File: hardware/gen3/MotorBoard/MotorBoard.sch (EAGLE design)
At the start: 245 parts, among them M10O1 TEST_PT, M1O2 TEST_PT, M1O3 TEST_PT, M2O1 TEST_PT, M2O2 TEST_PT, M2O3 TEST_PT, M3O1 TEST_PT, M3O2 TEST_PT, M3O3 TEST_PT, M4O1 TEST_PT, M4O2 TEST_PT, M4O3 TEST_PT, U2 ATMEGA165PV-8AU

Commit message: fixed weird package issues
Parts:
- C17, C35: device SparkFun-Passives:CAP1206 -> SparkFun-Passives:CAP0805
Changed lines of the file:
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@@
 <part name="R104" library="SparkFun-Resistors" deviceset="RESISTOR" device="0805-RES" value="37.5k"/>
 <part name="C8" library="SparkFun-Passives" deviceset="CAP" device="0805" value=".1uF"/>
-<part name="C17" library="SparkFun-Passives" deviceset="CAP" device="1206" value=".1uF"/>
+<part name="C17" library="SparkFun-Passives" deviceset="CAP" device="0805" value=".1uF"/>
 <part name="C26" library="SparkFun-Passives" deviceset="CAP" device="0805" value=".1uF"/>
-<part name="C35" library="SparkFun-Passives" deviceset="CAP" device="1206" value=".1uF"/>
+<part name="C35" library="SparkFun-Passives" deviceset="CAP" device="0805" value=".1uF"/>
 <part name="C44" library="SparkFun-Passives" deviceset="CAP" device="0805" value=".1uF"/>
 <part name="C45" library="SparkFun-Passives" deviceset="CAP" device="0805" value=".1uF"/>

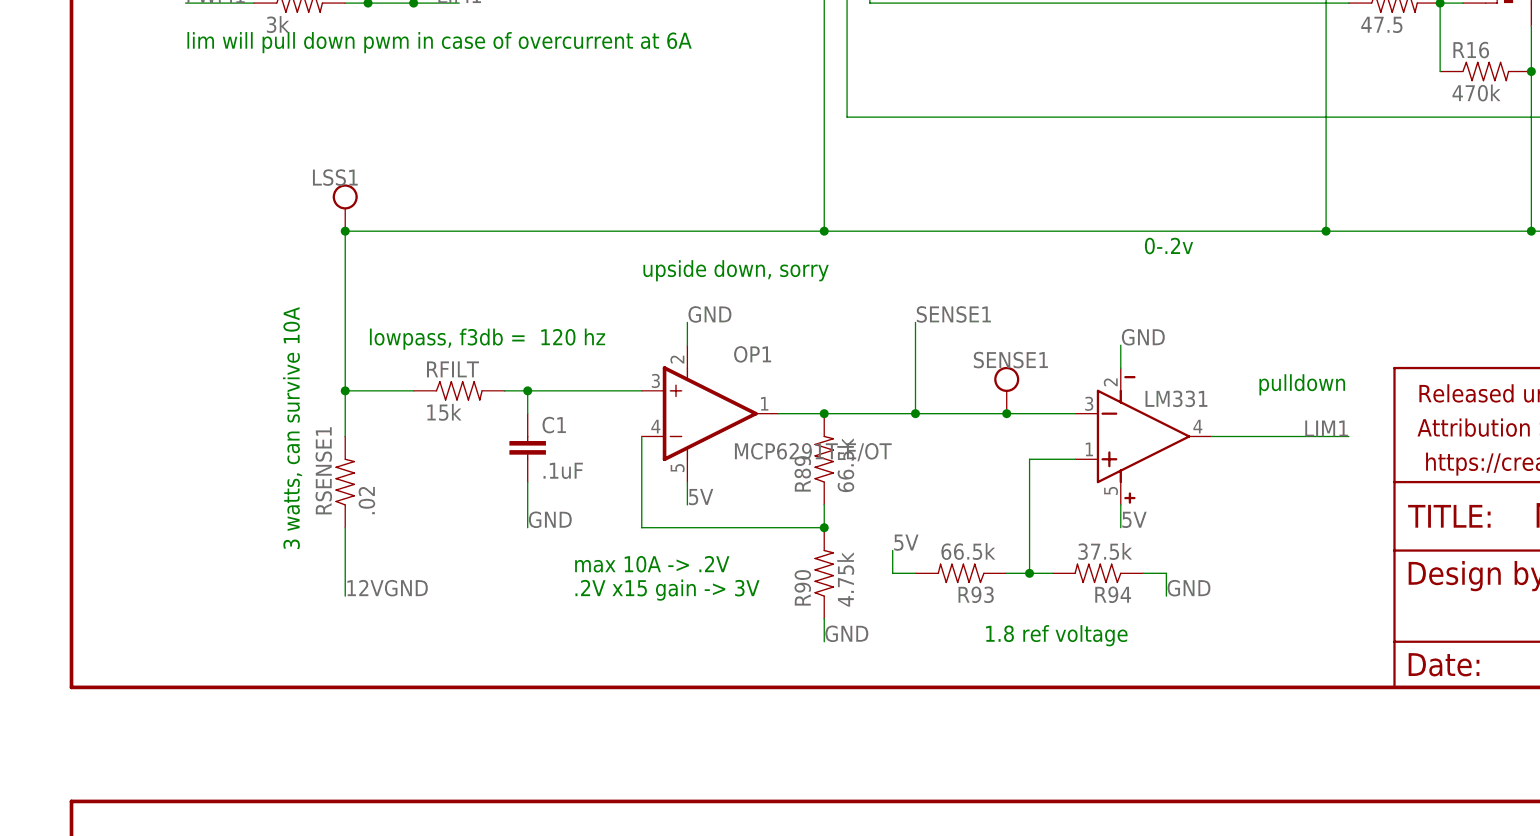
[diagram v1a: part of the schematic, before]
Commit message: schematic for differential amp
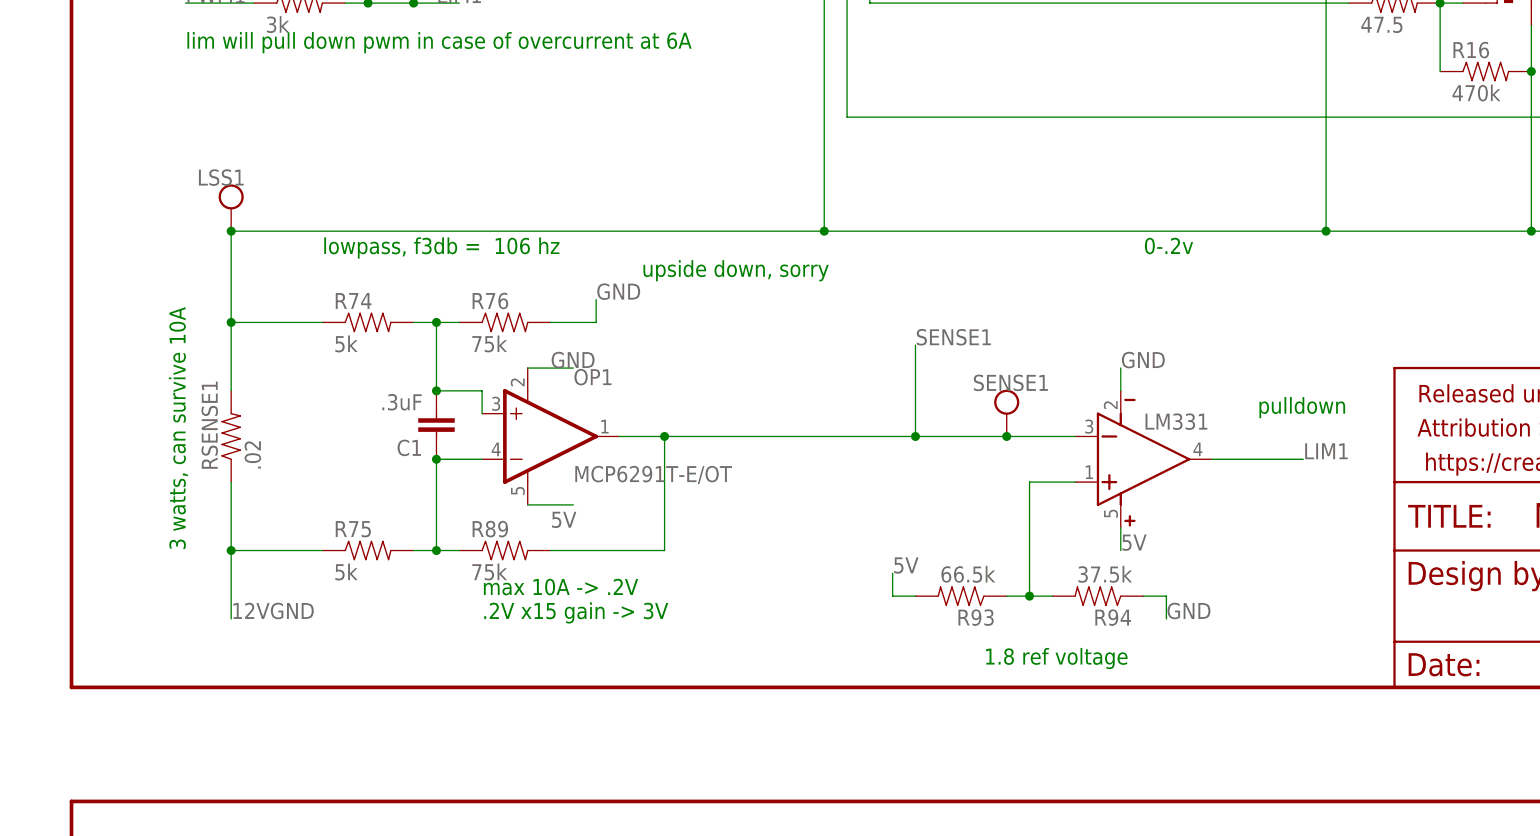
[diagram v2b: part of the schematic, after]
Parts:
- removed R90: 4.75k, SparkFun-Resistors:RESISTOR0805-RES
- removed RFILT: 15k, SparkFun-Resistors:RESISTOR0805-RES
- added R74, R75: 5k, SparkFun-Passives:RESISTOR0805-RES
- added R76: 75k, SparkFun-Passives:RESISTOR0805-RES
- C1: value .1uF -> .3uF
- R89: value 66.5k -> 75k; device SparkFun-Resistors:RESISTOR0805-RES -> SparkFun-Passives:RESISTOR0805-RES
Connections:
- removed net N$109: OP1.-IN, R89.1, R90.2
- new net N$92: C1.1, OP1.-IN, R75.2, R89.1
- net 12VGND: now also R75.1
- net GND: now also R76.2; no longer C1.2, R90.1
- net N$46: now also C1.2, R74.2, R76.1; no longer C1.1, RFILT.2
- net O1: now also R74.1; no longer RFILT.1
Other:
- note added: "lowpass, f3db = 106 hz"
- moved on the sheet: C1, LSS1, OP1, R89, R93, R94, RSENSE1, SENSE1
